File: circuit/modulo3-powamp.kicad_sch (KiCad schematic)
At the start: 47 parts, among them J1 HOLE, J2 HOLE, J3 HOLE, J4 HOLE, Q1 BS170, SW3 HEAD/AD, U1 DIFFAUDIO, U2 TPA3220, U5 PWR_CONN, U6 AMPCTRL

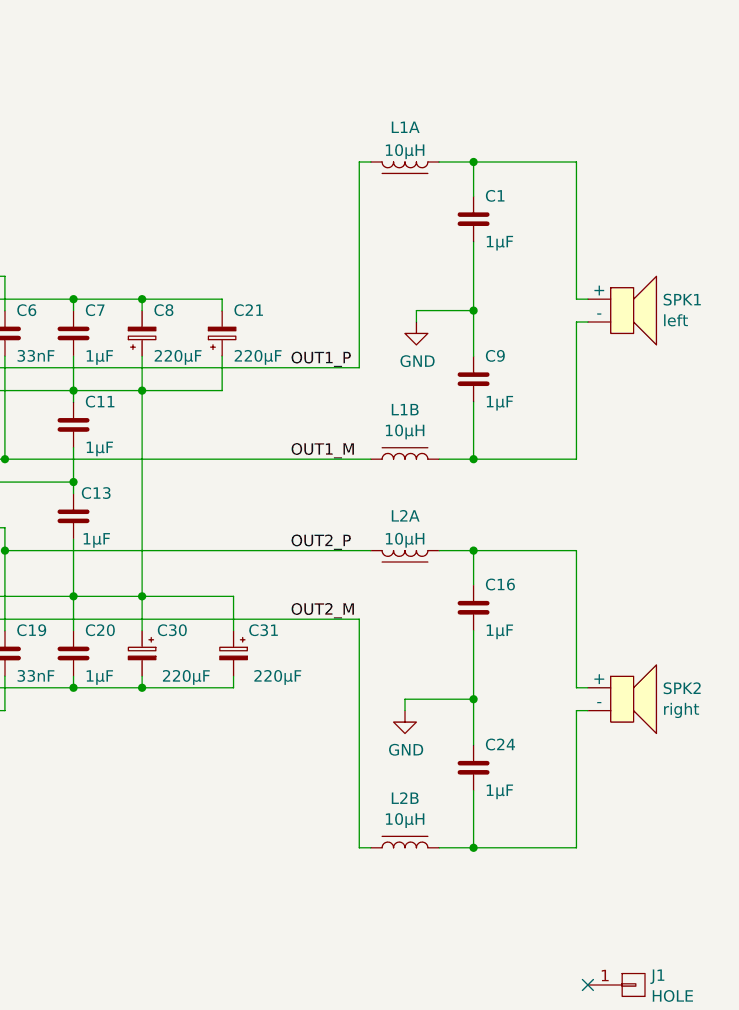
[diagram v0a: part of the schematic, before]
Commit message: fv-1 mostly done; power progressed
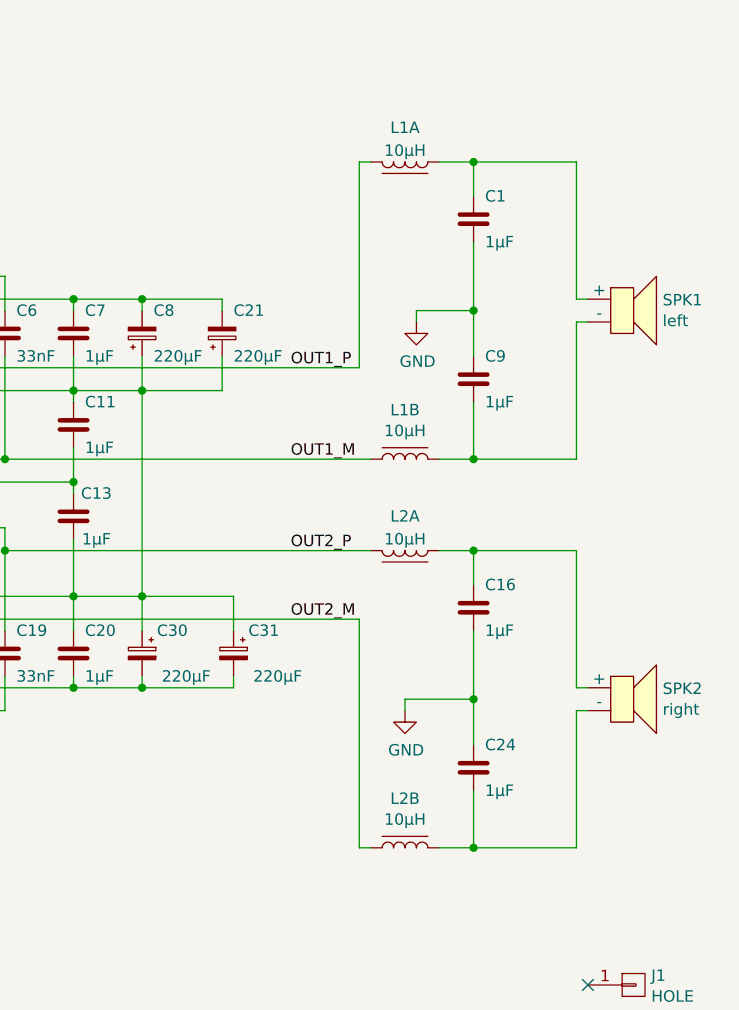
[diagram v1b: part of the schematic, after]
